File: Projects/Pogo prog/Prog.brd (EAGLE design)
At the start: 17.8 x 12.7 mm, 1 part, among them J1 RA 6Pin SMD

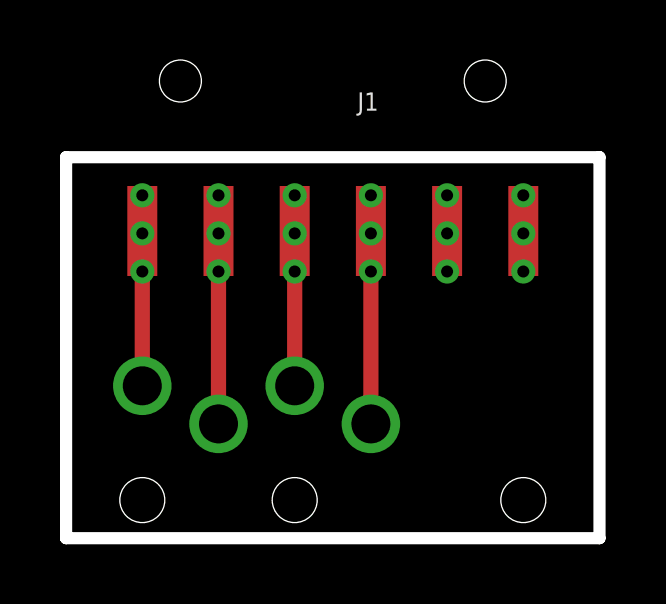
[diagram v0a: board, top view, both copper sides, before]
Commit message: Final design
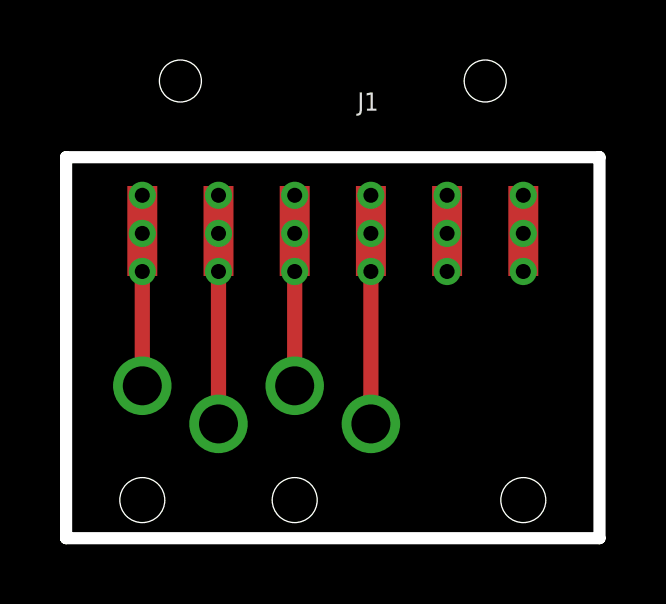
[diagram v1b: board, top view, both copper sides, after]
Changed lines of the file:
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@@
 <via x="6.35" y="46.99" extent="1-16" drill="1.3"/>
 <contactref element="J1" pad="6"/>
-<via x="6.35" y="53.34" extent="1-16" drill="0.4"/>
-<via x="6.35" y="52.07" extent="1-16" drill="0.4"/>
-<via x="6.35" y="50.8" extent="1-16" drill="0.4"/>
+<via x="6.35" y="53.34" extent="1-16" drill="0.5"/>
+<via x="6.35" y="52.07" extent="1-16" drill="0.5"/>
+<via x="6.35" y="50.8" extent="1-16" drill="0.5"/>
 <wire x1="6.35" y1="50.8" x2="6.35" y2="46.99" width="0.508" layer="1"/>
 <wire x1="6.35" y1="52.15" x2="6.35" y2="53.34" width="0" layer="19" extent="1-1"/>
@@
 <via x="8.89" y="45.72" extent="1-16" drill="1.3"/>
 <contactref element="J1" pad="5"/>
-<via x="8.89" y="50.8" extent="1-16" drill="0.4"/>
-<via x="8.89" y="52.07" extent="1-16" drill="0.4"/>
-<via x="8.89" y="53.34" extent="1-16" drill="0.4"/>
+<via x="8.89" y="50.8" extent="1-16" drill="0.5"/>
+<via x="8.89" y="52.07" extent="1-16" drill="0.5"/>
+<via x="8.89" y="53.34" extent="1-16" drill="0.5"/>
 <wire x1="8.89" y1="45.72" x2="8.89" y2="52.07" width="0.508" layer="1"/>
 <wire x1="8.89" y1="52.15" x2="8.89" y2="53.34" width="0" layer="19" extent="1-1"/>
@@
 <via x="13.97" y="45.72" extent="1-16" drill="1.3"/>
 <contactref element="J1" pad="3"/>
-<via x="13.97" y="53.34" extent="1-16" drill="0.4"/>
-<via x="13.97" y="52.07" extent="1-16" drill="0.4"/>
-<via x="13.97" y="50.8" extent="1-16" drill="0.4"/>
+<via x="13.97" y="53.34" extent="1-16" drill="0.5"/>
+<via x="13.97" y="52.07" extent="1-16" drill="0.5"/>
+<via x="13.97" y="50.8" extent="1-16" drill="0.5"/>
 <wire x1="13.97" y1="45.72" x2="13.97" y2="52.15" width="0.508" layer="1"/>
 <wire x1="13.97" y1="52.15" x2="13.97" y2="53.34" width="0" layer="19" extent="1-1"/>
@@
 <contactref element="J1" pad="4"/>
 <via x="11.43" y="46.99" extent="1-16" drill="1.3"/>
-<via x="11.43" y="53.34" extent="1-16" drill="0.4"/>
-<via x="11.43" y="52.07" extent="1-16" drill="0.4"/>
-<via x="11.43" y="50.8" extent="1-16" drill="0.4"/>
+<via x="11.43" y="53.34" extent="1-16" drill="0.5"/>
+<via x="11.43" y="52.07" extent="1-16" drill="0.5"/>
+<via x="11.43" y="50.8" extent="1-16" drill="0.5"/>
 <wire x1="11.43" y1="46.99" x2="11.43" y2="52.15" width="0.508" layer="1"/>
 <wire x1="11.43" y1="52.15" x2="11.43" y2="53.34" width="0" layer="19" extent="1-1"/>
@@
 </signal>
 <signal name="N$15">
-<via x="16.51" y="53.34" extent="1-16" drill="0.4"/>
+<via x="16.51" y="53.34" extent="1-16" drill="0.5"/>
 </signal>
 <signal name="N$16">
-<via x="16.51" y="52.07" extent="1-16" drill="0.4"/>
+<via x="16.51" y="52.07" extent="1-16" drill="0.5"/>
 </signal>
 <signal name="N$17">
-<via x="16.51" y="50.8" extent="1-16" drill="0.4"/>
+<via x="16.51" y="50.8" extent="1-16" drill="0.5"/>
 </signal>
 <signal name="N$18">
-<via x="19.05" y="53.34" extent="1-16" drill="0.4"/>
+<via x="19.05" y="53.34" extent="1-16" drill="0.5"/>
 </signal>
 <signal name="N$19">
-<via x="19.05" y="52.07" extent="1-16" drill="0.4"/>
+<via x="19.05" y="52.07" extent="1-16" drill="0.5"/>
 </signal>
 <signal name="N$20">
-<via x="19.05" y="50.8" extent="1-16" drill="0.4"/>
+<via x="19.05" y="50.8" extent="1-16" drill="0.5"/>
 </signal>
 </signals>
